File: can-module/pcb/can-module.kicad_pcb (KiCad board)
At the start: 2 copper layers, 25.4 x 19 mm, 31 parts, among them IC1 PIC32CM1216JH01048-I_U5B, J1 Conn_01x08_Socket, J2 Conn_01x02_Socket, J3 Conn_01x04_Socket, U1 ATA6560-GBQW-N

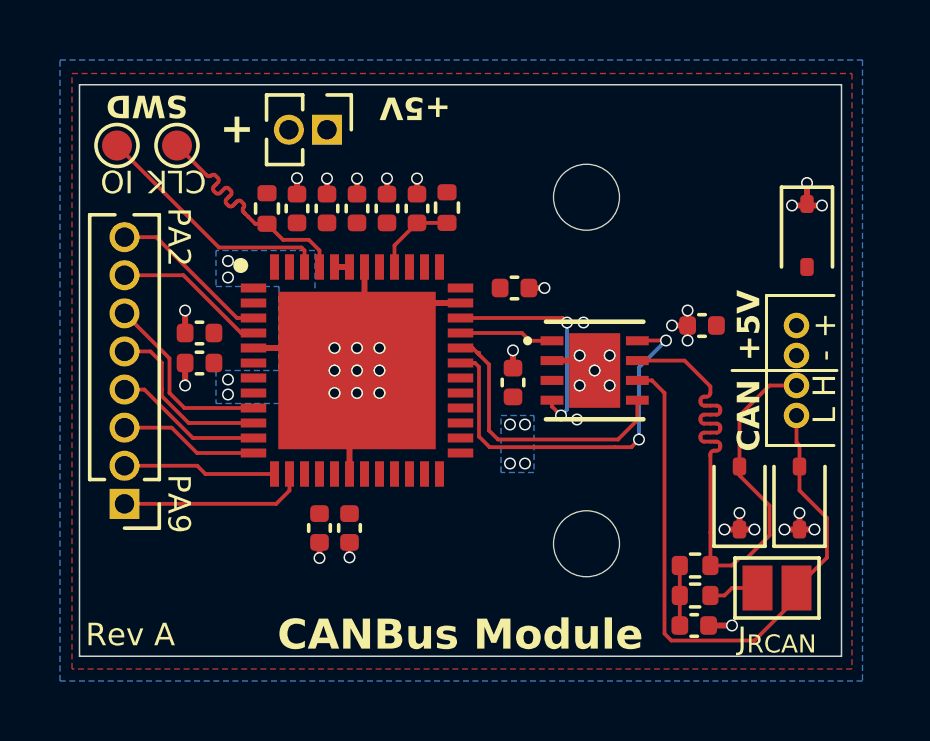
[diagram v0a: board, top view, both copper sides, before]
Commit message: can-module: Resolve hole clearance issue
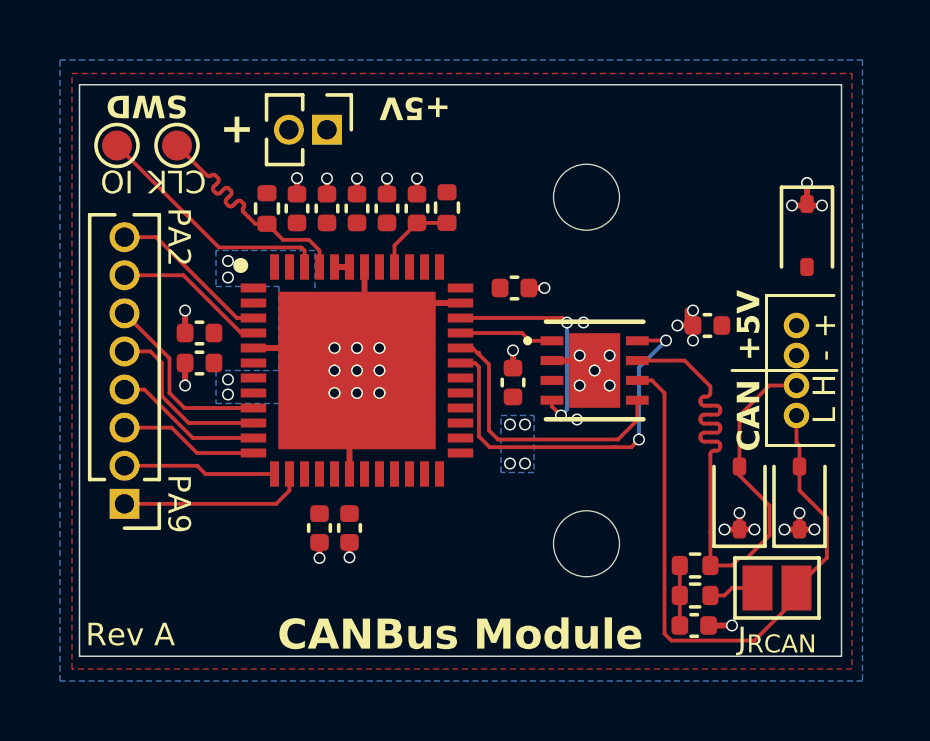
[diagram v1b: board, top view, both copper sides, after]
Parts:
- moved C12 0.18 mm to (133.7, 57.5)
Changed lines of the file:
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@@
 	(footprint "Capacitor_SMD:C_0402_1005Metric"
 		(layer "F.Cu")
-		(at 133.5 57.525 180)
+		(at 133.68 57.525 180)
 		(descr "Capacitor SMD 0402 (1005 Metric), square (rectangular) end terminal, IPC-7351 nominal, (Body size source: IPC-SM-782 page 76, https://www.pcb-3d.com/wordpress/wp-content/uploads/ipc-sm-782a_amendment_1_and_2.pdf), generated with kicad-footprint-generator")
 		(tags "capacitor")
@@
 	)
 	(segment
-		(start 133.02 57.525)
-		(end 133.02 58.025)
+		(start 133.2 57.525)
+		(end 133.2 58.025)
 		(width 0.2)
 		(layer "F.Cu")
@@
 	)
 	(segment
-		(start 133.02 57.525)
-		(end 132.5 57.525)
+		(start 133.2 57.525)
+		(end 132.68 57.525)
 		(width 0.2)
 		(layer "F.Cu")
@@
 	)
 	(via
-		(at 133.02 57.025)
+		(at 133.2 57.025)
 		(size 0.4)
 		(drill 0.3)
@@
 	)
 	(via
-		(at 133.02 58.025)
+		(at 133.2 58.025)
 		(size 0.4)
 		(drill 0.3)
@@
 	)
 	(via
-		(at 132.5 57.525)
+		(at 132.68 57.525)
 		(size 0.4)
 		(drill 0.3)
@@
 		(single_sided no)
 		(target_length 8.2509)
-		(target_length_max 8.3509)
+		(target_length_max 8.350899)
 		(target_length_min 8.1509)
 		(target_skew 0)
